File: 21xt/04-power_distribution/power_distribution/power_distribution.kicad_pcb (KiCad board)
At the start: 4 copper layers, 27 parts, among them J1 Conn_01x02, J3 Conn_01x02, J4 Conn_01x02, Q2 NVMFWS2D1N08XT1G, Q3 NVMFWS2D1N08XT1G, U2 XIAO-ESP32-C3-DIP, U3 LM74700, U4 LM74700, U5 LTC2959, U6 TLV76150DCY

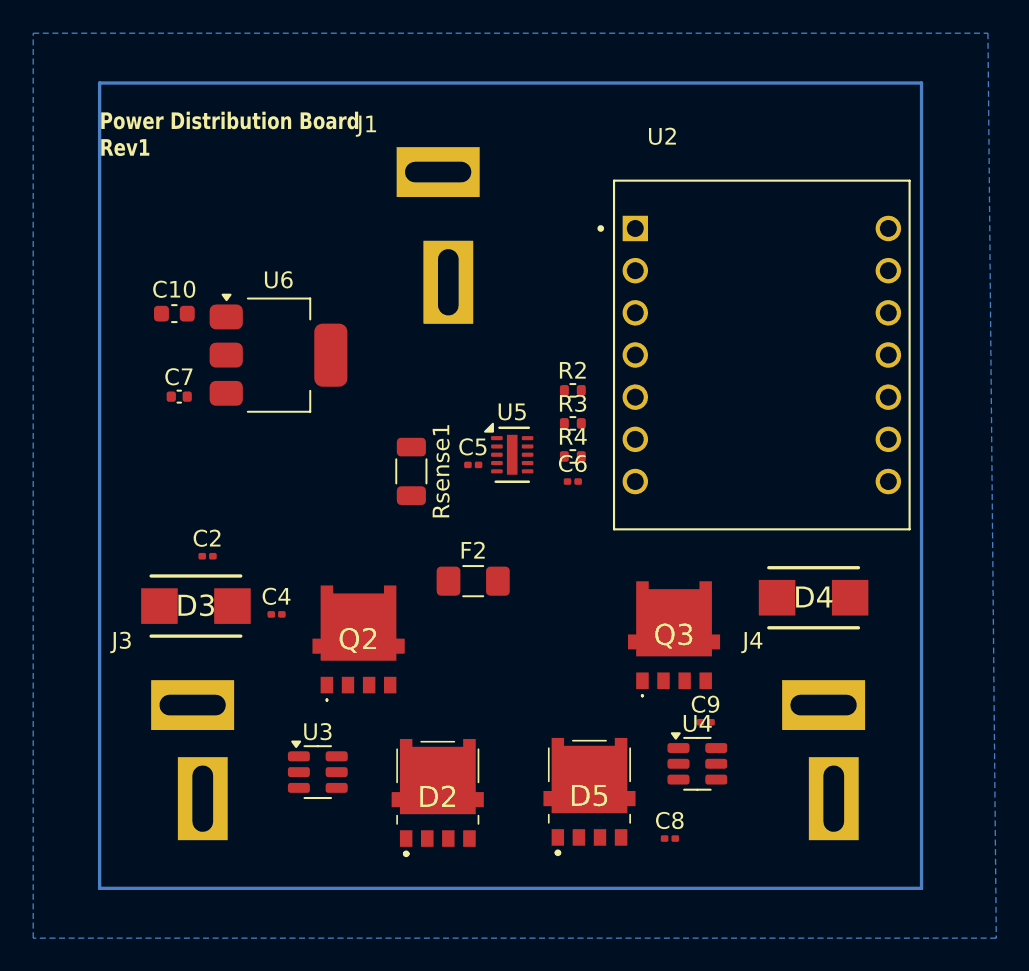
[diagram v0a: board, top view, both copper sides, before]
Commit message: PCB layed out
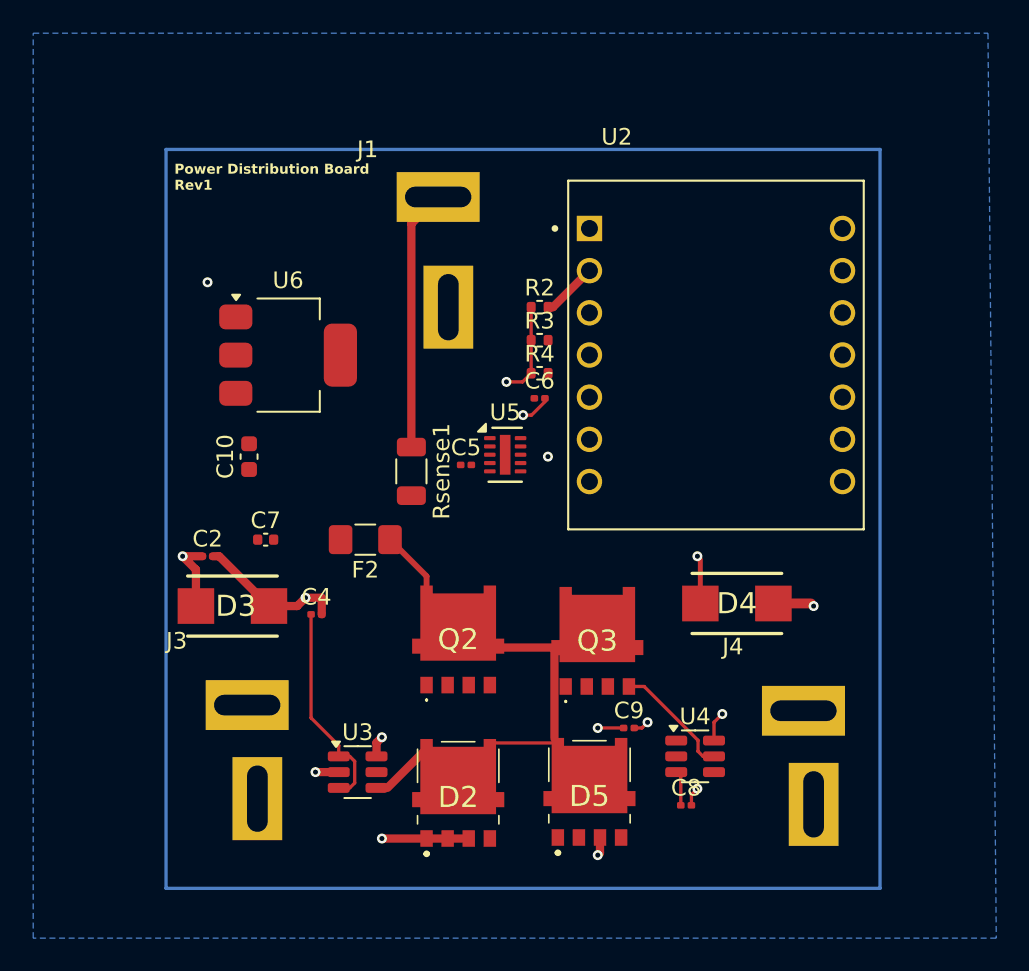
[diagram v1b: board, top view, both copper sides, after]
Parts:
- moved C7 10.1 mm to (114.0, 111.0)
- moved C10 9.72 mm to (113.0, 106.0), turned to 90 degrees
- moved F2 6.96 mm to (120.0, 111.0), turned to 180 degrees
- moved Q2 6.00 mm to (125.6, 117.0)
- moved C6 5.39 mm to (130.5, 102.5)
- moved R2 5.39 mm to (130.5, 97.0)
- moved R3 5.39 mm to (130.5, 99.0)
- moved R4 5.39 mm to (130.5, 101.0)
- moved C9 4.63 mm to (135.9, 122.3)
- moved D4 4.63 mm to (142.4, 114.8)
- moved Q3 4.63 mm to (134.0, 117.1)
- moved J3 3.29 mm to (108.6, 117.6)
- moved U2 2.76 mm to (141.1, 99.9)
- moved C4 2.40 mm to (117.1, 115.5)
- moved U3 2.40 mm to (119.5, 125.0)
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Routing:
- net Battery1_Supply: track 0.00 -> 21.5 mm
- net Net-(J1-Pin_1): track 0.00 -> 15.7 mm
- net Battery2: track 0.00 -> 15.5 mm, vias 0 -> 3
- net Net-(U3-EN): track 0.00 -> 12.7 mm
- net GND: track 0.00 -> 12.2 mm, vias 0 -> 6
- net Battery1: track 0.00 -> 7.51 mm, vias 0 -> 5
- net Net-(Q3-G): track 0.00 -> 7.25 mm
- net 3V3 ESP32: track 0.00 -> 5.69 mm, vias 0 -> 2
- net Net-(U2-GPIO3/A1/D1): track 0.00 -> 3.40 mm
- net Net-(U4-EN): track 0.00 -> 2.11 mm
- added copper zone on In2.Cu, net Battery1
